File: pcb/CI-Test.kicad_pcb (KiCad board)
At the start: 2 copper layers, 20 x 20 mm, 4 parts, among them J1 Conn_01x01, J2 Conn_01x01

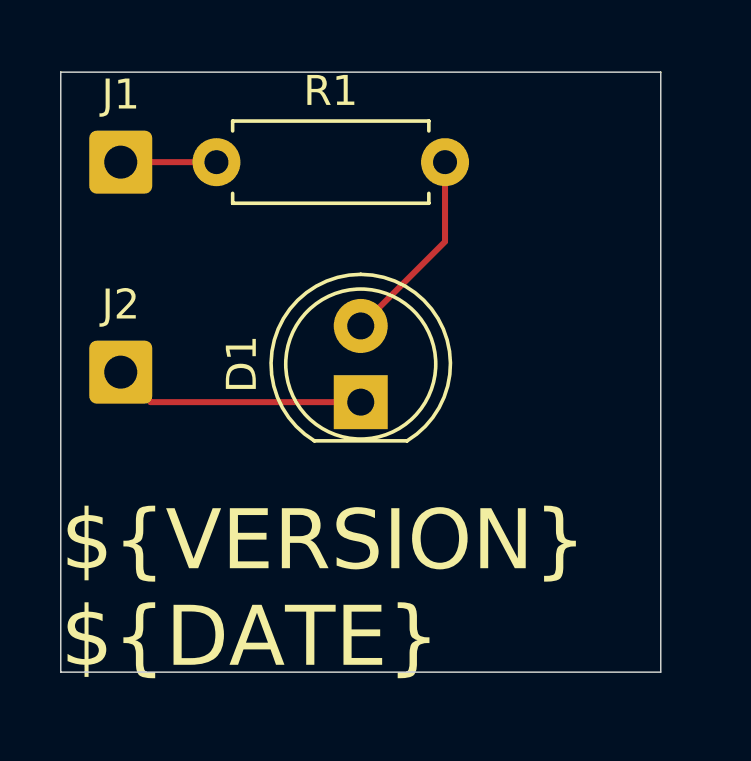
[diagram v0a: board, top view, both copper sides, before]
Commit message: fix: testfix
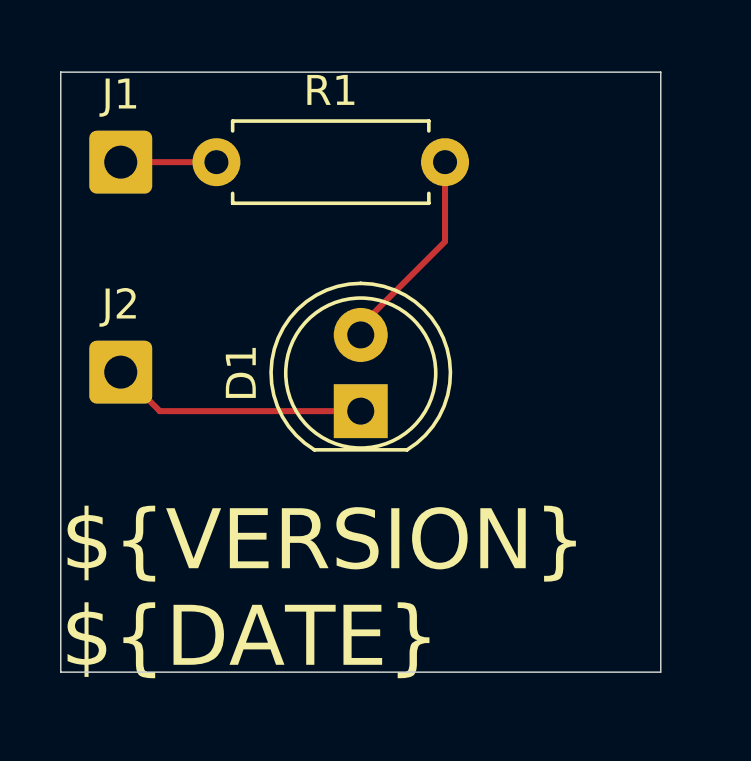
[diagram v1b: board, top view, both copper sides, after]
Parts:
- moved D1 0.30 mm to (150.0, 91.3)
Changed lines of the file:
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@@
 	(footprint "LED_THT:LED_D5.0mm"
 		(layer "F.Cu")
-		(at 150 91 90)
+		(at 150 91.3 90)
 		(descr "LED, diameter 5.0mm, 2 pins, http://cdn-reichelt.de/documents/datenblatt/A500/LL-504BC2E-009.pdf")
 		(tags "LED diameter 5.0mm 2 pins")
@@
 	)
 	(segment
-		(start 150 91)
-		(end 143 91)
+		(start 143.3 91.3)
+		(end 142 90)
 		(width 0.2)
 		(layer "F.Cu")
@@
 	)
 	(segment
-		(start 143 91)
-		(end 142 90)
+		(start 150 91.3)
+		(end 143.3 91.3)
 		(width 0.2)
 		(layer "F.Cu")
